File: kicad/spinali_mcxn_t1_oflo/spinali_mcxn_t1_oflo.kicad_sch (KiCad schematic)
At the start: 0 parts

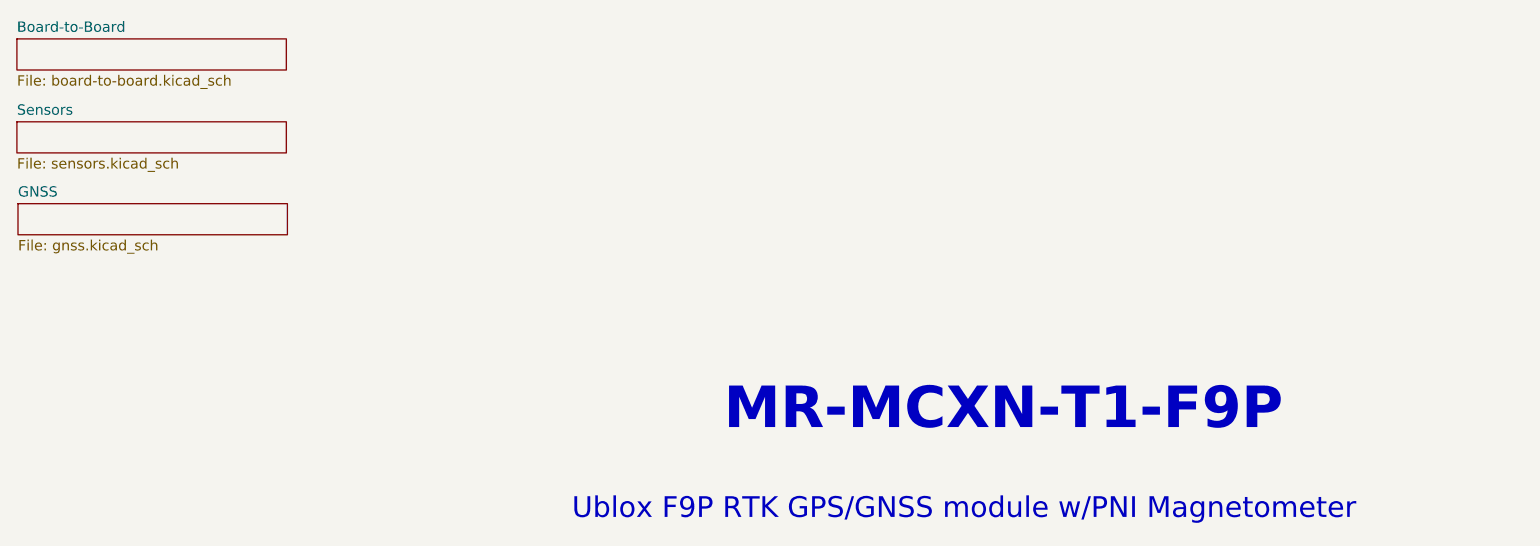
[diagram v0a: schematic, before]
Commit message: Finish rename and org.
Signed-off-by: Benjamin Perseghetti <bperseghetti@rudislabs.com>
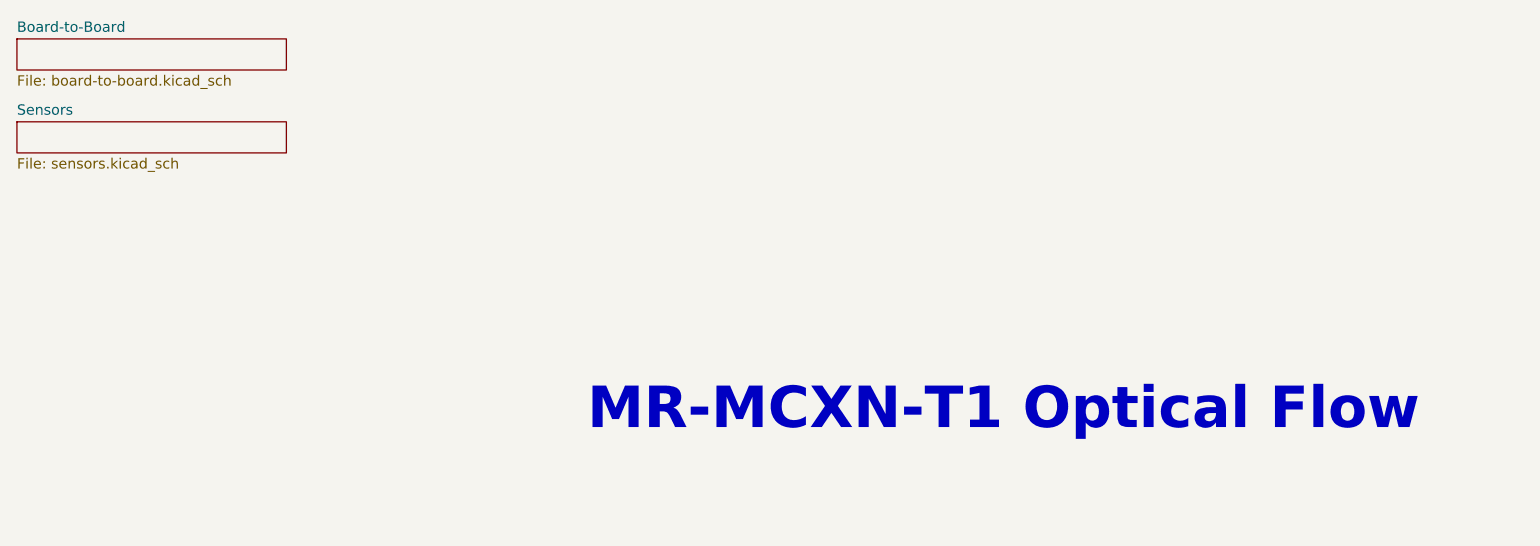
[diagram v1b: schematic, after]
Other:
- removed sheet GNSS
- note added: "MR-MCXN-T1 Optical Flow"
- note removed: "${TITLE}"
- note removed: "Ublox F9P RTK GPS/GNSS module w/PNI Magnetometer"
- title: MR-MCXN-T1-F9P -> MR-MCXN-T1-OFLO
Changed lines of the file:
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@@
 	(paper "A4")
 	(title_block
-		(title "MR-MCXN-T1-F9P")
-		(date "2025-08-27")
-		(rev "X1")
+		(title "MR-MCXN-T1-OFLO")
+		(date "2025-04-16")
+		(rev "X0")
 		(company "NXP SEMICONDUCTORS B.V.")
-		(comment 1 "CLASSIFICATION: INTERNAL USE ONLY")
-		(comment 3 "DESIGNER: YOURI TILS, Iain Galloway")
+		(comment 3 "DESIGNER: YOURI TILS")
 		(comment 4 "CTO SYSTEM INNOVATIONS / MOBILE ROBOTICS DOMAIN")
 	)
-	(text "Ublox F9P RTK GPS/GNSS module w/PNI Magnetometer"
-		(exclude_from_sim no)
-		(at 145.288 104.648 0)
-		(effects
-			(font
-				(size 2.54 2.54)
-			)
-		)
-	)
-	(text "${TITLE}"
+	(text "MR-MCXN-T1 Optical Flow"
 		(exclude_from_sim no)
 		(at 150.114 92.456 0)
@@
 				(thickness 1.016)
 				(bold yes)
-			)
-		)
-	)
-	(sheet
-		(at 29.337 67.183)
-		(size 33.02 3.81)
-		(exclude_from_sim no)
-		(in_bom yes)
-		(on_board yes)
-		(dnp no)
-		(fields_autoplaced yes)
-		(stroke
-			(width 0.1524)
-			(type solid)
-		)
-		(fill
-			(color 0 0 0 0.0000)
-		)
-		(property "Sheetname" "GNSS"
-			(at 29.337 66.4714 0)
-			(effects
-				(font
-					(size 1.27 1.27)
-				)
-				(justify left bottom)
-			)
-		)
-		(property "Sheetfile" "gnss.kicad_sch"
-			(at 29.337 71.5776 0)
-			(effects
-				(font
-					(size 1.27 1.27)
-				)
-				(justify left top)
-			)
-		)
-		(instances
-			(project "spinali_add-on_GNSS_F9P"
-				(path "/04285d74-eeba-483c-9378-52bd287e15a2"
-					(page "4")
-				)
 			)
 		)
@@
 		)
 		(instances
-			(project "spinali_add-on_GNSS_F9P"
+			(project "spinali_mcxn_t1_oflo"
 				(path "/04285d74-eeba-483c-9378-52bd287e15a2"
 					(page "2")
@@
 		)
 		(instances
-			(project "spinali_add-on_GNSS_F9P"
+			(project "spinali_mcxn_t1_oflo"
 				(path "/04285d74-eeba-483c-9378-52bd287e15a2"
 					(page "3")
